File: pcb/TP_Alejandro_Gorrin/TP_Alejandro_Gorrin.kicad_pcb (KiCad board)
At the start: 2 copper layers, 33 parts, among them J1 Conn_01x12, J2 Conn_01x02, J3 Conn_01x16, J4 USB_A, Q1 MMBT3904, Q2 MMBT3904, Q3 BS250, SW1 SW_1, U1 MCP73831-2-OT, U3 CP2104, U4 AP2112K-3.3, U5 ESP3212

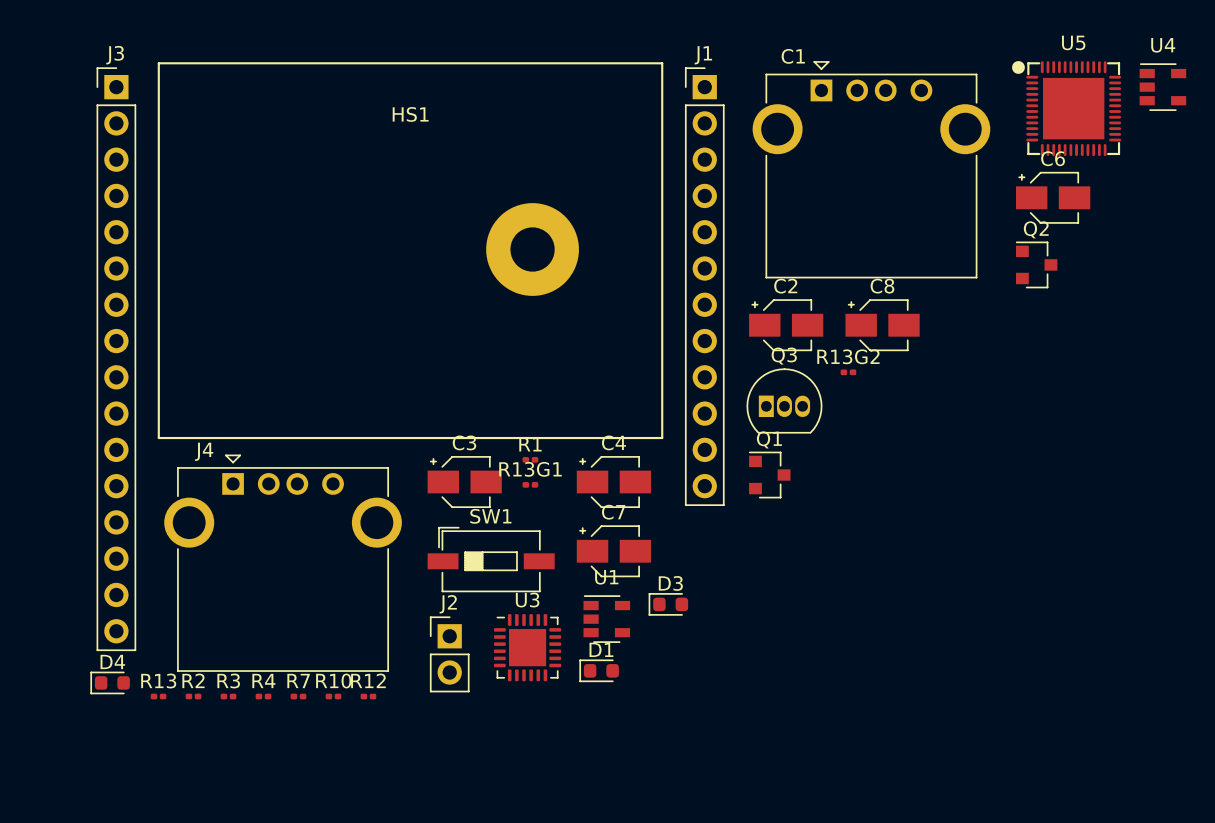
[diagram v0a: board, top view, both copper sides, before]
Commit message: Empezando con el ruteo
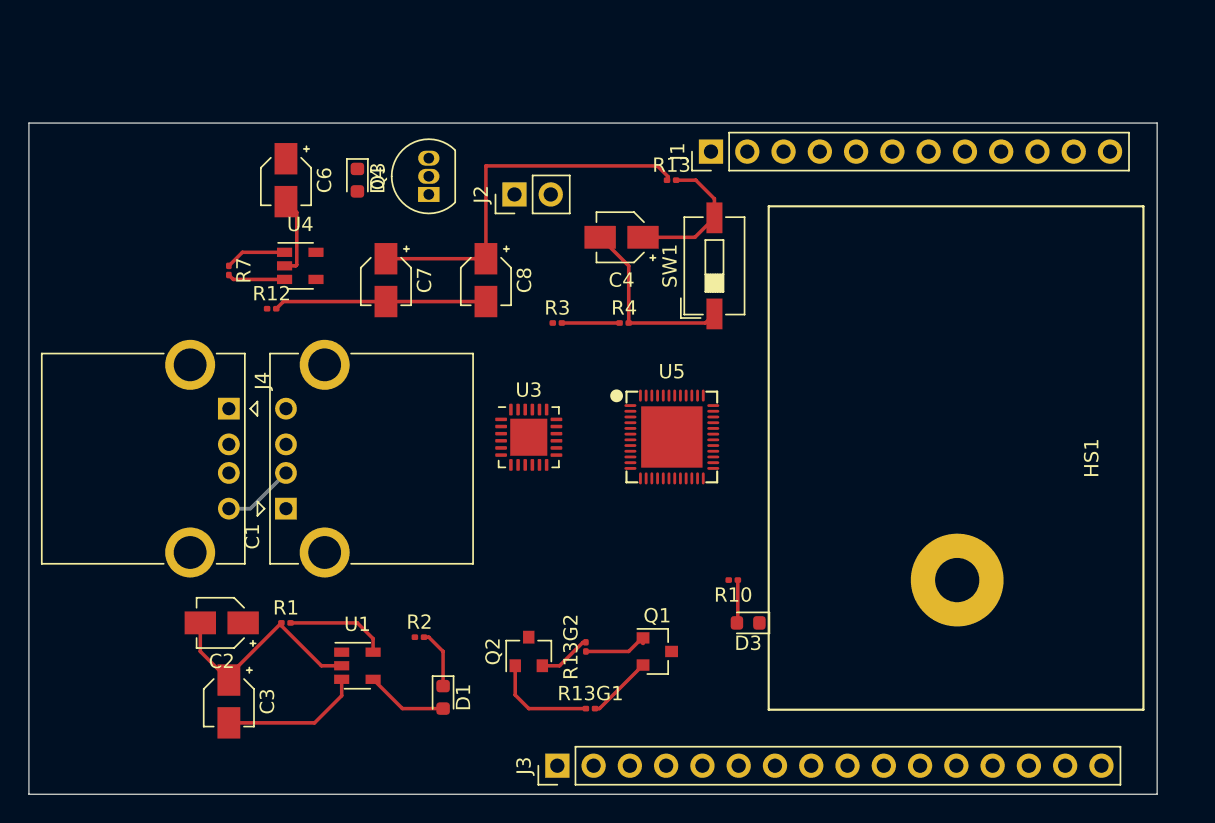
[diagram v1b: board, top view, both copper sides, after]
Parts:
- moved U4 61.7 mm to (129.0, 88.0)
- moved J3 56.7 mm to (147.0, 123.0), turned to 90 degrees
- moved C6 53.7 mm to (128.0, 82.0), turned to 270 degrees
- moved R13 51.0 mm to (155.0, 82.0)
- moved C1 47.6 mm to (128.0, 105.0), turned to 90 degrees
- moved Q2 44.7 mm to (145.0, 115.0), turned to 90 degrees
- moved C2 44.7 mm to (123.5, 113.0), turned to 180 degrees
- moved D4 39.2 mm to (133.0, 82.0), turned to 270 degrees
- moved HS1 37.7 mm to (175.0, 110.0), turned to 270 degrees
- moved R4 36.4 mm to (151.7, 92.0)
- moved U5 36.3 mm to (155.0, 100.0)
- moved R3 34.8 mm to (147.0, 92.0)
- moved J2 31.3 mm to (144.0, 83.0), turned to 90 degrees
- moved R7 30.2 mm to (124.0, 88.3), turned to 270 degrees
- moved R10 29.2 mm to (159.3, 110.0), turned to 180 degrees
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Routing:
- net GNDD: track 0.00 -> 54.6 mm
- net +3V3: track 0.00 -> 26.9 mm
- net /RESET: track 0.00 -> 10.2 mm
- net +BATT: track 0.00 -> 9.84 mm
- net Net-(Q2-Pad1): track 0.00 -> 7.39 mm
- net Net-(R1-Pad2): track 0.00 -> 7.19 mm
- net VBUS: track 0.00 -> 5.75 mm
- net Net-(Q1-Pad1): track 0.00 -> 5.23 mm
- net /RTS: track 0.00 -> 4.62 mm
- net Net-(C6-Pad1): track 0.00 -> 4.29 mm
- net Net-(D1-Pad1): track 0.00 -> 4.17 mm
- net /A13_I35: track 0.00 -> 4.04 mm
- net Net-(R7-Pad2): track 0.00 -> 4.03 mm
- net /DTR: track 0.00 -> 3.73 mm
- net Net-(D3-Pad2): track 0.00 -> 3.03 mm
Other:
- board outline added: 79 x 47 mm
- net class Prueba added: clearance 0.8, trace_width 0.8, via_dia 1.6, via_drill 0.8
